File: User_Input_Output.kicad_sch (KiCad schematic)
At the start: 42 parts, among them SW10 SW_DIP_x01, SW2 SW_DIP_x01, SW3 SW_DIP_x01, SW4 SW_DIP_x01, SW5 SW_DIP_x01, SW6 SW_DIP_x01, SW7 SW_DIP_x01, SW8 SW_DIP_x01, SW9 SW_DIP_x01

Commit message: Add files via upload
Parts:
- R15, R16, R2: footprint Resistor_SMD:R_1206_3216Metric_Pad1.30x1.75mm_HandSolder -> Resistor_SMD:R_0805_2012Metric_Pad1.20x1.40mm_HandSolder
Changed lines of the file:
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@@
       (effects (font (size 1.27 1.27)) (justify left))
     )
-    (property "Footprint" "Resistor_SMD:R_1206_3216Metric_Pad1.30x1.75mm_HandSolder" (at 199.517 144.78 90)
+    (property "Footprint" "Resistor_SMD:R_0805_2012Metric_Pad1.20x1.40mm_HandSolder" (at 199.517 144.78 90)
       (effects (font (size 1.27 1.27)) hide)
     )
@@
       (effects (font (size 1.27 1.27)) (justify left))
     )
-    (property "Footprint" "Resistor_SMD:R_1206_3216Metric_Pad1.30x1.75mm_HandSolder" (at 208.407 147.955 90)
+    (property "Footprint" "Resistor_SMD:R_0805_2012Metric_Pad1.20x1.40mm_HandSolder" (at 208.407 147.955 90)
       (effects (font (size 1.27 1.27)) hide)
     )
@@
       (effects (font (size 1.27 1.27)) (justify left))
     )
-    (property "Footprint" "Resistor_SMD:R_1206_3216Metric_Pad1.30x1.75mm_HandSolder" (at 271.907 147.955 90)
-      (effects (font (size 1.27 1.27)) hide)
-    )
+    (property "Footprint" "Resistor_SMD:R_0805_2012Metric_Pad1.20x1.40mm_HandSolder" (at 271.907 147.955 90)
+      (effects (font (size 1.27 1.27)) hide)
+    )

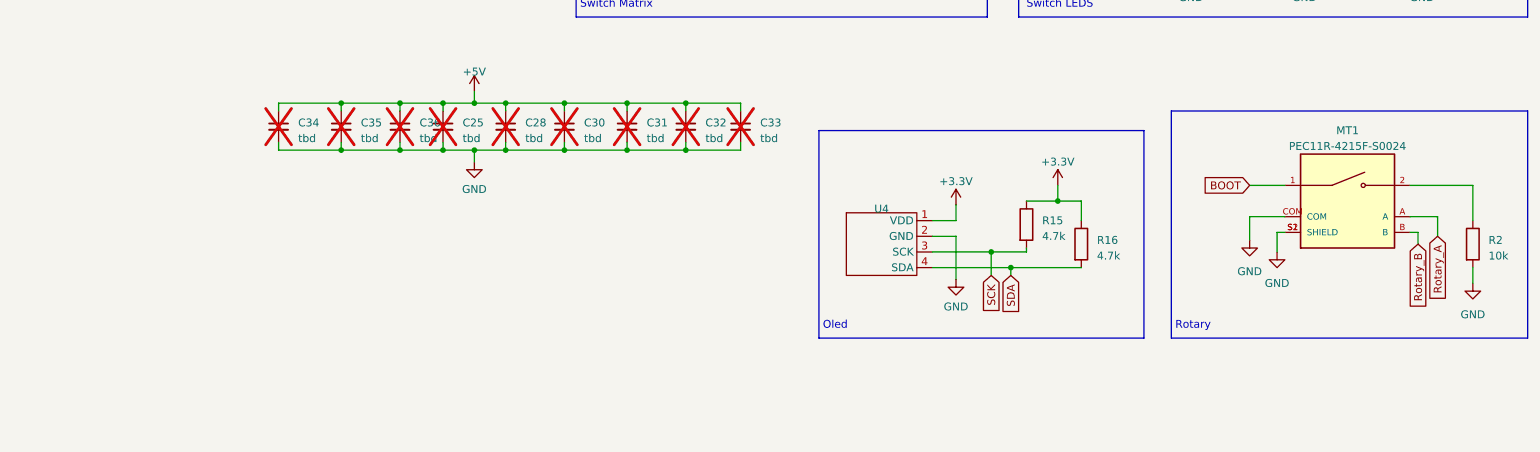
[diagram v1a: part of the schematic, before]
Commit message: Add files via upload
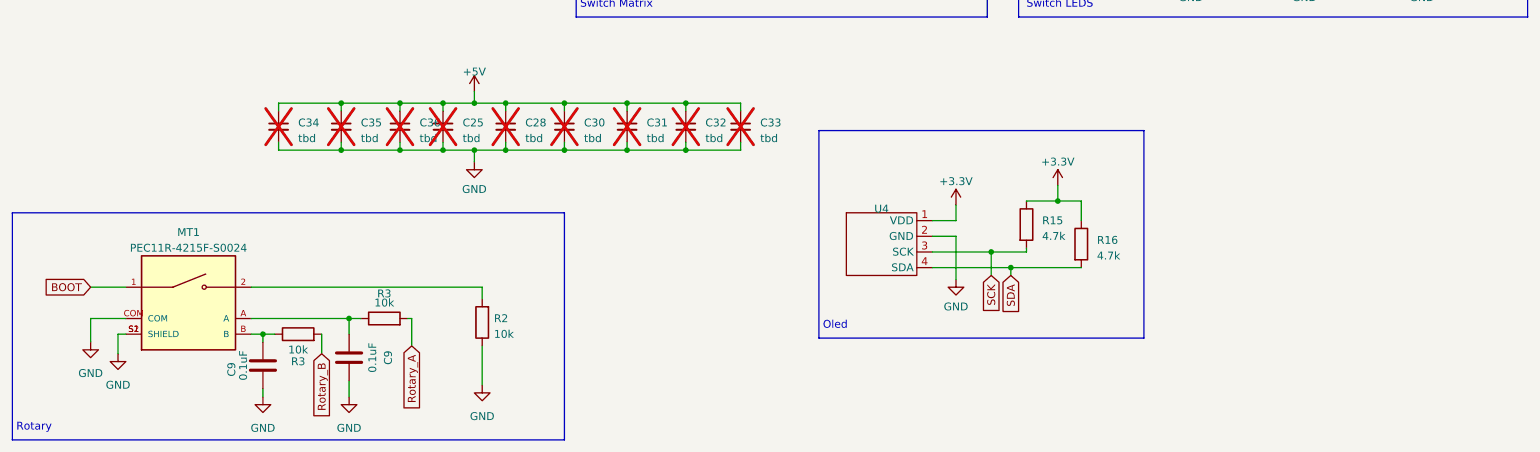
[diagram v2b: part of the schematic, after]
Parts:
- added C9 (x2): 0.1uF, Capacitor_SMD:C_0603_1608Metric_Pad1.08x0.95mm_HandSolder, symbol Device:C
- added R3 (x2): 10k, Resistor_SMD:R_0805_2012Metric_Pad1.20x1.40mm_HandSolder, symbol Device:R
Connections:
- net GND: now also R2.1, C9.2, C9.2; no longer R2.2
- net Rotary_A: now also R3.2; no longer MT1.A
- net Rotary_B: now also R3.2; no longer MT1.B
- net at MT1.2: now also R2.2; no longer R2.1
- new net: C9.1, MT1.A, R3.1
- new net: C9.1, MT1.B, R3.1
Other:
- moved on the sheet: MT1, R2
